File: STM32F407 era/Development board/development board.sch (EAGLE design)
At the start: 75 parts, among them IC1 74HC595N, IC2 74HC595N, IC3 317T, IC4 317T, U1 MAX13052ESA+, X1 K375M, X2 HD44780LCD-1602, X3 SDBMF, X4 057-006-1, X8 057-006-1, X9 057-006-1

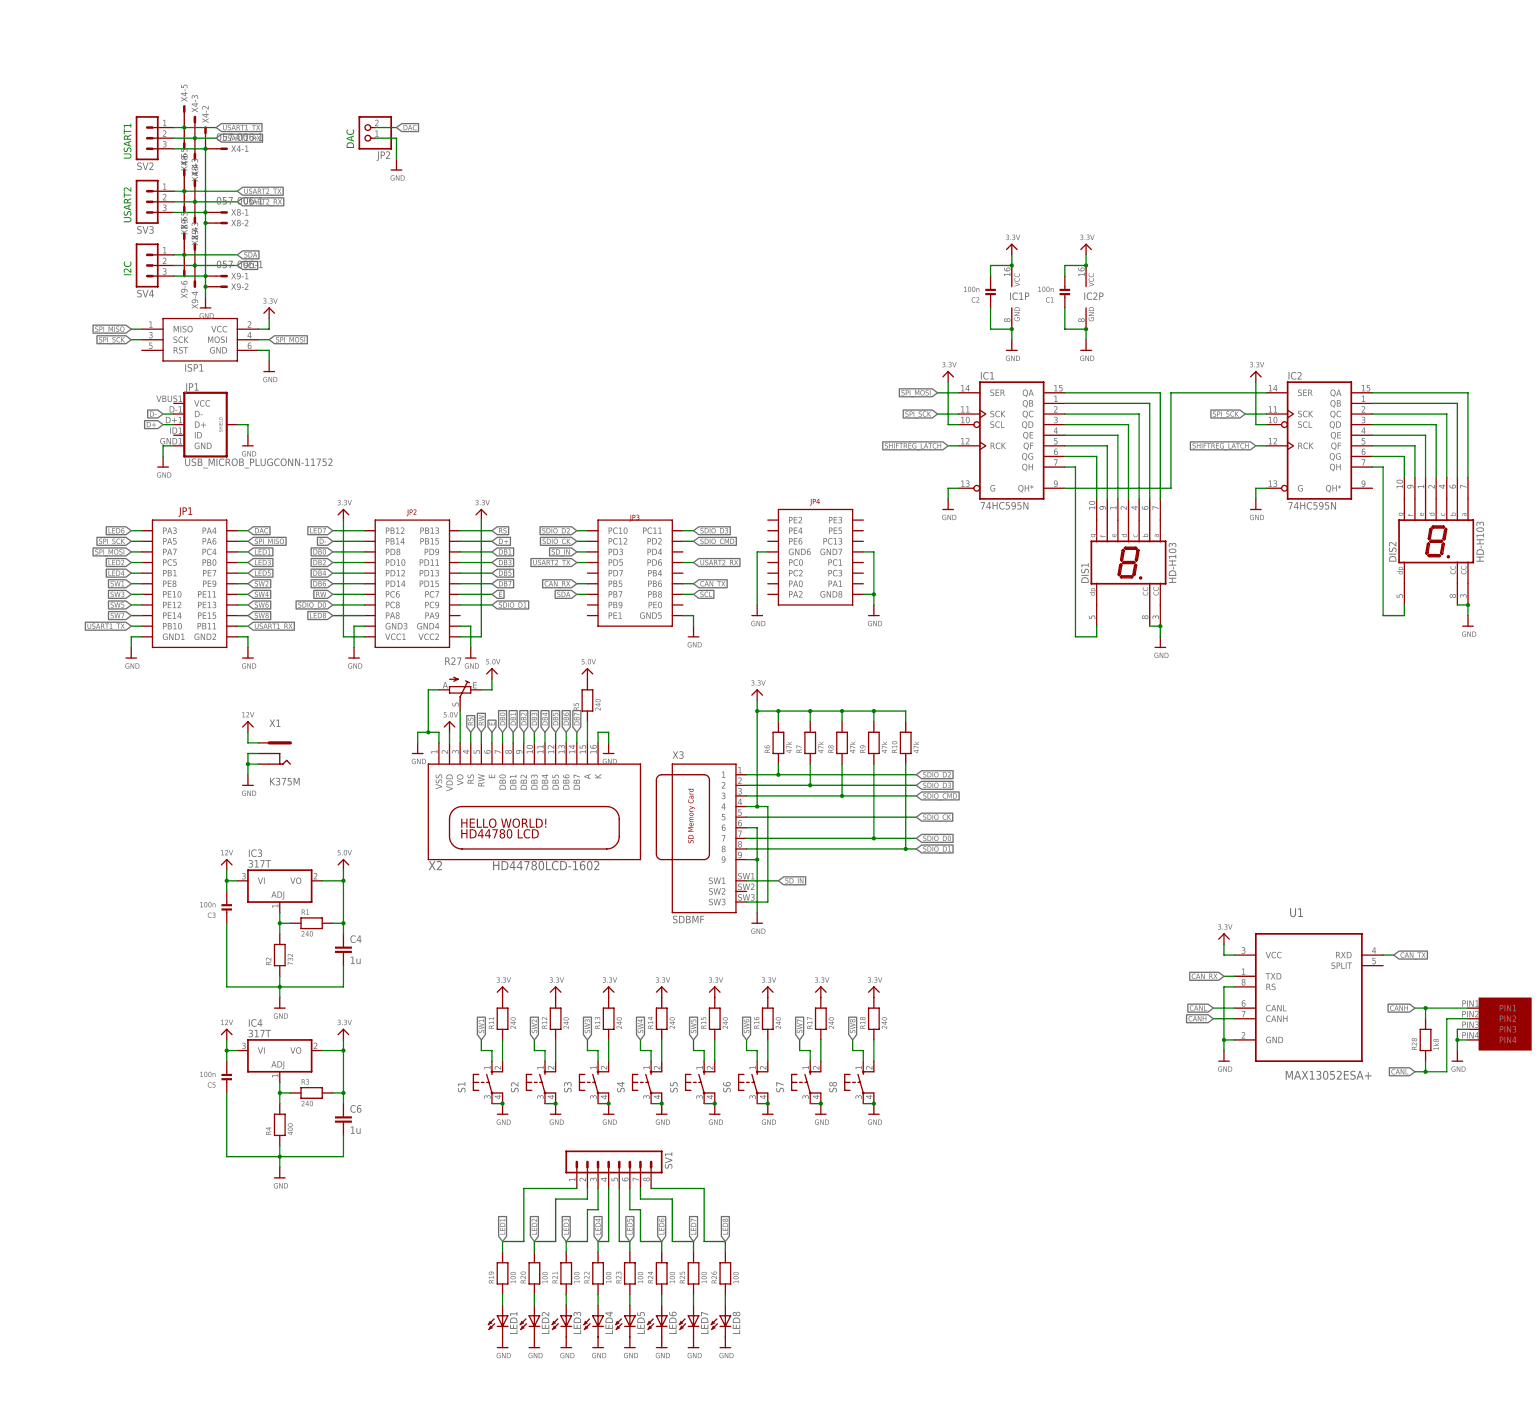
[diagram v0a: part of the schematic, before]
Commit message: updates to the layout and done routing (maybe)
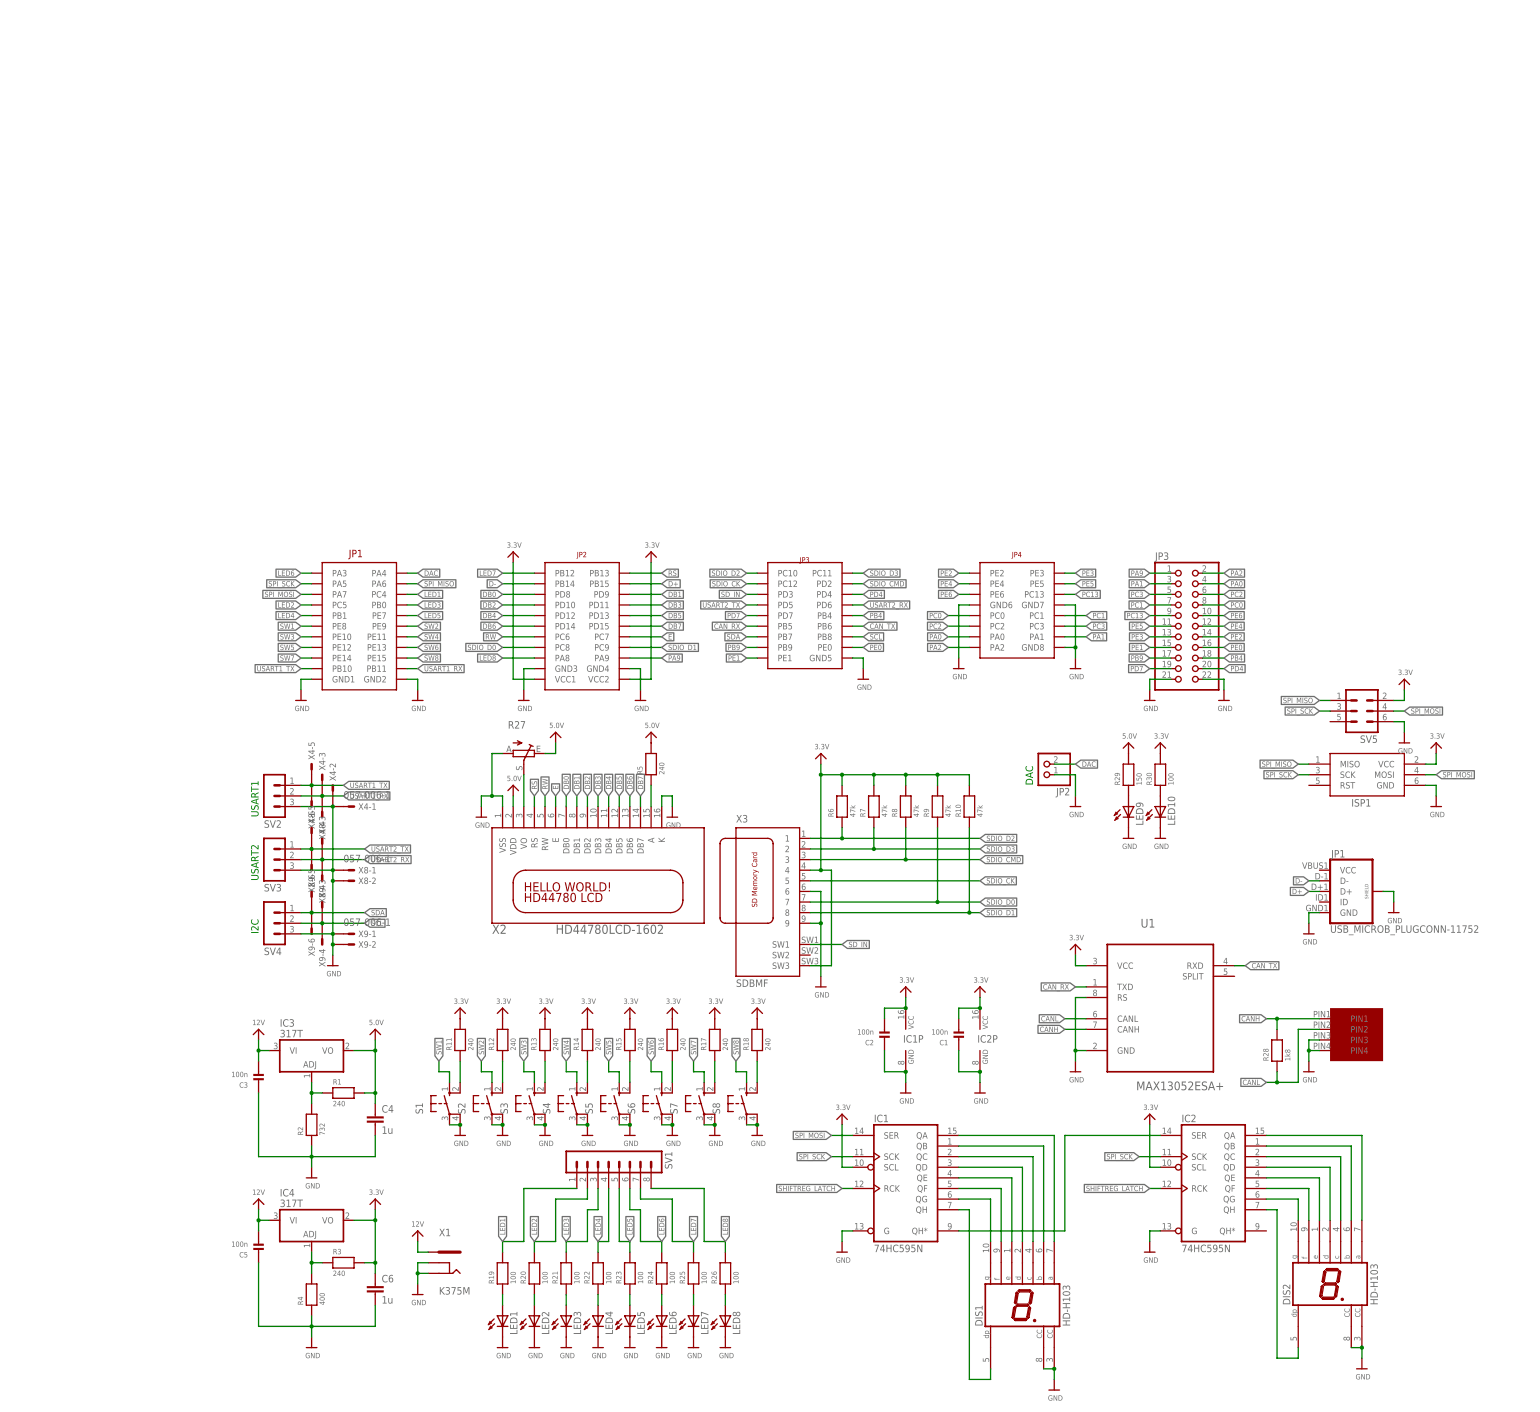
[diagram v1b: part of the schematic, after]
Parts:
- added JP3: (no value), pinhead:PINHD-2X11
- added LED10, LED9: (no value), led:LED3MM
- added R29: 150, microbuilder:RESISTOR_0603
- added R30: 100, microbuilder:RESISTOR_0603
- added SV5: (no value), con-lstb:MA03-2
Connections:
- new net N$20: LED10.A, R30.1
- new net N$31: LED9.A, R29.1
- new net PA0: JP3.4, U$1G$4.PA0
- new net PA1: JP3.3, U$1G$4.PA1
- new net PA2: JP3.2, U$1G$4.PA2
- new net PA9: JP3.1, U$1G$2.PA9
- new net PB4: JP3.18, U$1G$3.PB4
- new net PB9: JP3.17, U$1G$3.PB9
- new net PC0: JP3.8, U$1G$4.PC0
- new net PC1: JP3.7, U$1G$4.PC1
- new net PC13: JP3.9, U$1G$4.PC13
- new net PC2: JP3.6, U$1G$4.PC2
- new net PC3: JP3.5, U$1G$4.PC3
- new net PD4: JP3.20, U$1G$3.PD4
- new net PD7: JP3.19, U$1G$3.PD7
- new net PE0: JP3.16, U$1G$3.PE0
- new net PE1: JP3.15, U$1G$3.PE1
- new net PE2: JP3.14, U$1G$4.PE2
- new net PE3: JP3.13, U$1G$4.PE3
- new net PE4: JP3.12, U$1G$4.PE4
- new net PE5: JP3.11, U$1G$4.PE5
- new net PE6: JP3.10, U$1G$4.PE6
- net 3.3V: now also R30.2, SV5.2
- net 5.0V: now also R29.2
- net GND: now also JP3.21, JP3.22, LED10.C, LED9.C, SV5.6
- net SPI_MISO: now also SV5.1
- net SPI_MOSI: now also SV5.4
- net SPI_SCK: now also SV5.3
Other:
- moved on the sheet: C1, C2, C3, C4, C5, C6, DIS1, DIS2, IC1, IC1P, IC2, IC2P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
